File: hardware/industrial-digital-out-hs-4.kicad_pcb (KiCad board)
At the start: 2 copper layers, 40 x 40 mm, 49 parts, among them P1 CON-SENSOR, P2 Digital Output, P3 Debug, P4 Boot, Q1 FDS8449, U1 XMC1100, U2 VN7140AS, U3 VN7140AS, U4 VN7140AS, U5 VN7140AS, U6 DRILL, U7 DRILL, U8 DRILL, U9 DRILL

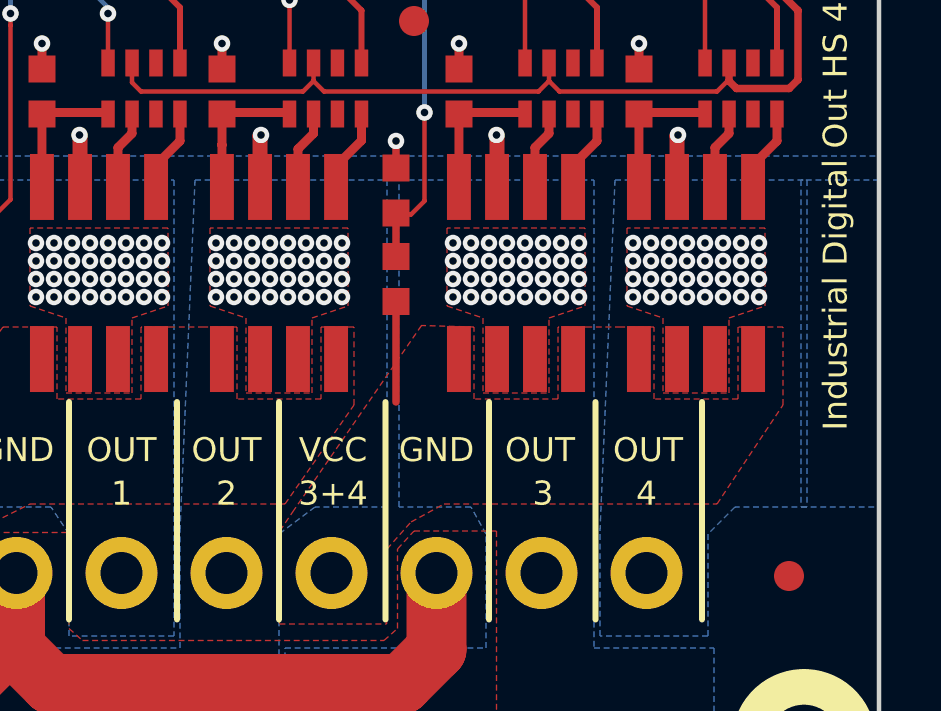
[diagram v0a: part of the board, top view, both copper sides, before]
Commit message: drc check
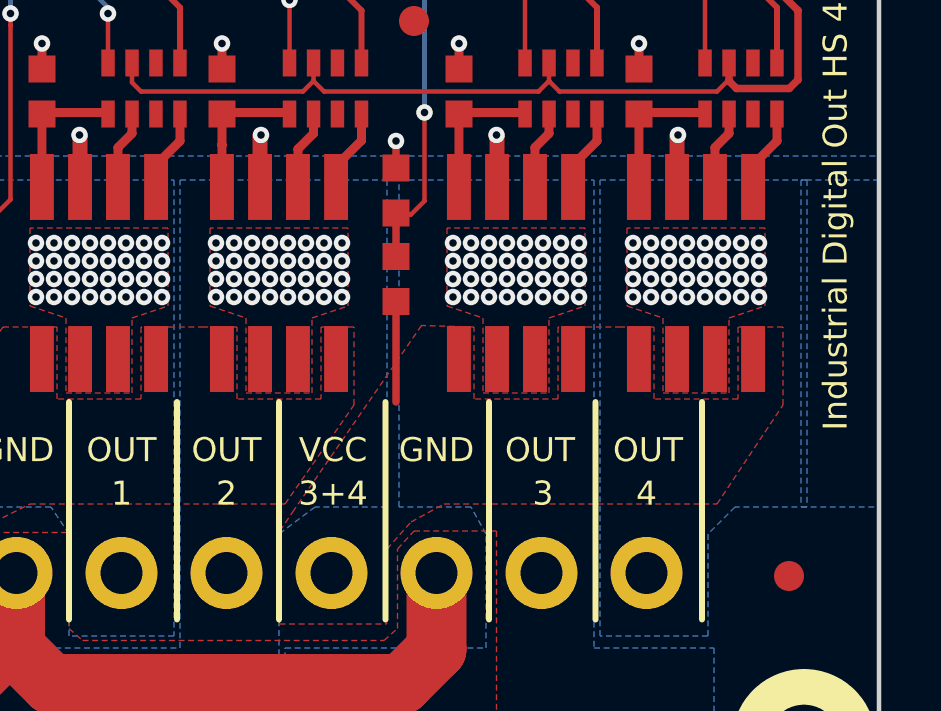
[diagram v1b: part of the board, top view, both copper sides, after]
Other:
- net class Default: clearance 0.19 -> 0.149
- rule pad_to_mask_clearance: 0.051 -> 0
- rule trace_clearance: 0.19 -> 0.149
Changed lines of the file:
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@@
     (user_trace_width 2)
     (user_trace_width 3)
-    (trace_clearance 0.19)
+    (trace_clearance 0.149)
     (zone_clearance 0.2)
     (zone_45_only no)
@@
     (pad_size 1.4 1.4)
     (pad_drill 0.6)
-    (pad_to_mask_clearance 0.051)
-    (solder_mask_min_width 0.25)
+    (pad_to_mask_clearance 0)
     (aux_axis_origin 118 73)
     (grid_origin 118 73)
@@
     (pcbplotparams
       (layerselection 0x010fc_ffffffff)
-      (usegerberextensions false)
+      (usegerberextensions true)
       (usegerberattributes false)
       (usegerberadvancedattributes false)
@@
       (plotinvisibletext false)
       (padsonsilk false)
-      (subtractmaskfromsilk false)
+      (subtractmaskfromsilk true)
       (outputformat 1)
       (mirror false)
-      (drillshape 1)
+      (drillshape 0)
       (scaleselection 1)
-      (outputdirectory ""))
+      (outputdirectory "proto/"))
   )
   (net 0 "")
@@
   (net 52 "Net-(RP5-Pad5)")
   (net_class Default "Dies ist die voreingestellte Netzklasse."
-    (clearance 0.19)
+    (clearance 0.149)
     (trace_width 0.25)
     (via_dia 0.8)
@@
       (pts
         (xy 141.6 102.7) (xy 139.2 102.7) (xy 138 103.6) (xy 138 112.55) (xy 123.5 112.55)
-        (xy 123.5 107.4) (xy 134.7 107.4) (xy 134.7 103.5) (xy 135.2 91.8) (xy 141.6 91.8)
+        (xy 123.5 107.4) (xy 134.7 107.4) (xy 134.7 103.5) (xy 134.7 91.8) (xy 141.6 91.8)
       )
     )
@@
     (polygon
       (pts
-        (xy 149.2 91.8) (xy 155.6 91.8) (xy 155.6 102.7) (xy 153.2 102.7) (xy 152.3 103.6)
+        (xy 148.7 91.8) (xy 155.6 91.8) (xy 155.6 102.7) (xy 153.2 102.7) (xy 152.3 103.6)
         (xy 152.3 107) (xy 148.7 107) (xy 148.7 103.5)
       )
